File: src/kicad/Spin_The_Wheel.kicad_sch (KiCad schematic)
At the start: 42 parts, among them J1 USB_A, Q1 NPN, Q2 NPN, Q3 NPN, Q5 PNP, Q6 PNP, SW1 START, SW2 STOP, U1 ICM7555xB, U2 4017

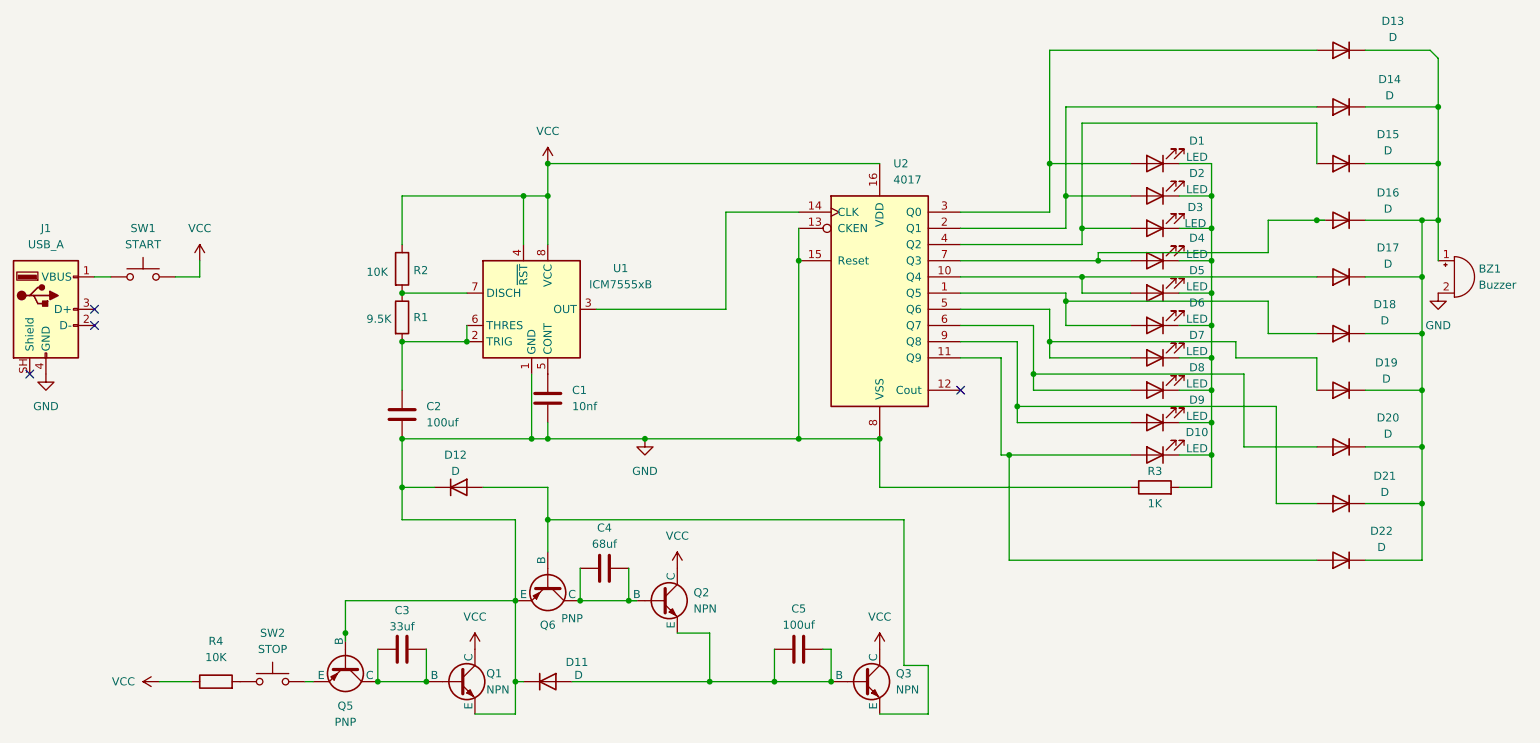
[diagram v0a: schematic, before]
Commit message: Add files via upload
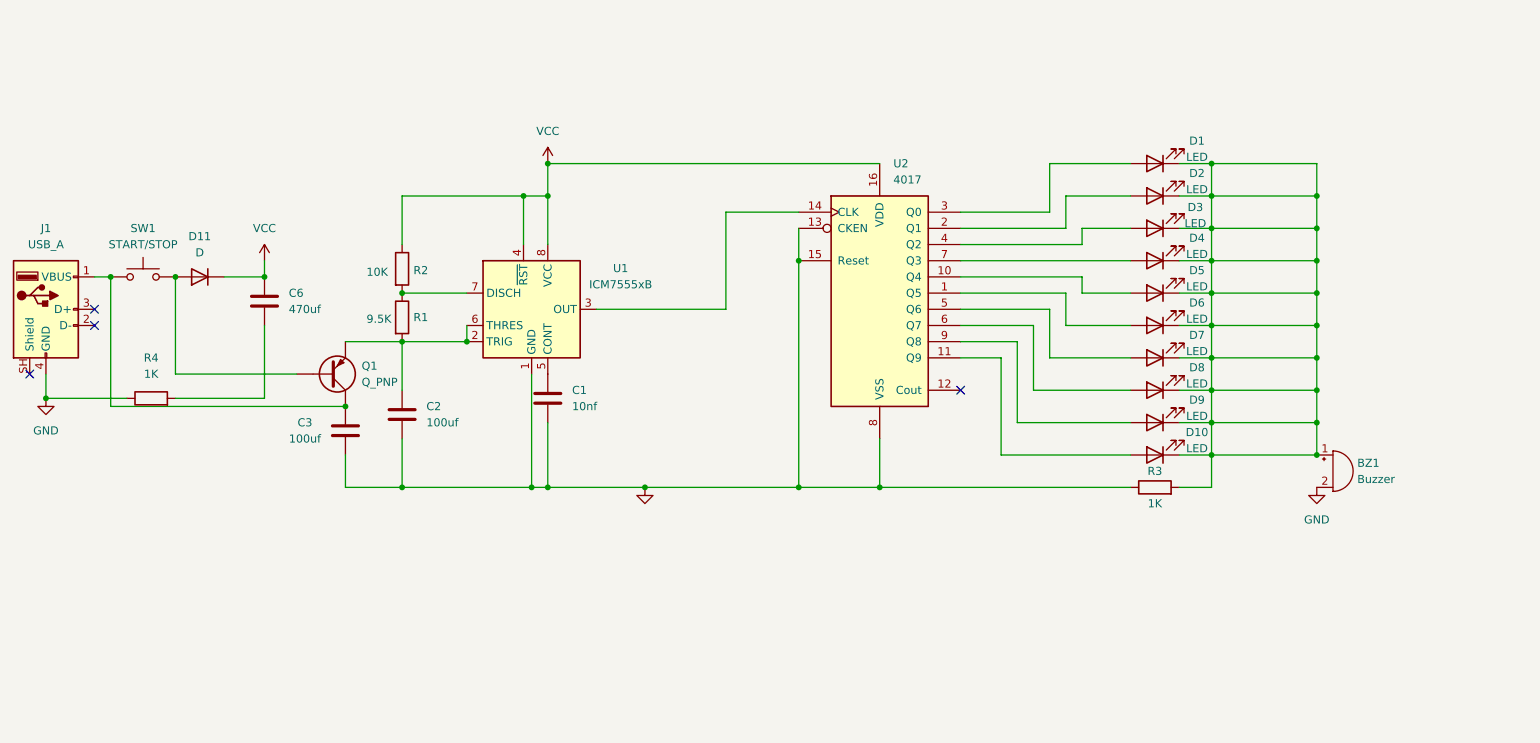
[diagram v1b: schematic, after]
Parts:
- removed C4: 68uf, Capacitor_THT:C_Disc_D8.0mm_W5.0mm_P5.00mm, symbol Device:C
- removed C5: 100uf, Capacitor_THT:C_Disc_D8.0mm_W5.0mm_P5.00mm, symbol Device:C
- removed D12: D, Diode_THT:D_DO-15_P15.24mm_Horizontal, symbol Device:D
- removed D13, D14, D15, D16, D17, D18, D19, D20, D21, D22: D, Diode_THT:D_DO-15_P15.24mm_Horizontal, symbol Diode:1N914
- removed Q1, Q2, Q3: NPN, Package_TO_SOT_THT:TO-92L_Inline_Wide, symbol Simulation_SPICE:NPN
- removed Q5, Q6: PNP, Package_TO_SOT_THT:TO-92L_Inline_Wide, symbol Simulation_SPICE:PNP
- removed SW2: STOP, Button_Switch_THT:SW_PUSH-12mm, symbol Switch:SW_Push
- added C6: 470uf, Capacitor_THT:C_Disc_D8.0mm_W5.0mm_P5.00mm, symbol Device:C
- added Q1: Q_PNP, Package_TO_SOT_THT:TO-92L_Inline_Wide, symbol Device:Q_PNP
- C3: value 33uf -> 100uf
- R4: value 10K -> 1K
- SW1: value START -> START/STOP
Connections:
- net GND: now also C3.1, R4.1; no longer D11.1 (K)
- net VCC: now also D11.1 (K), C6.1; no longer R4.1, SW1.2
- net at BZ1.1 (+): now also D1.1 (K), D10.1 (K), D2.1 (K), D3.1 (K), D4.1 (K), D5.1 (K), D6.1 (K), D7.1 (K), D8.1 (K), D9.1 (K), R3.2
- net at C2.1, R1.2, U1.2 (TRIG)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: now also Q1.E
- net at D11.2 (A): now also SW1.2, Q1.B
- net at C3.2: now also J1.1 (VBUS), SW1.1, Q1.C; no longer C3.1
- net at R4.2: now also C6.2
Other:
- moved on the sheet: BZ1, C3
